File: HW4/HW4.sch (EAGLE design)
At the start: 27 parts

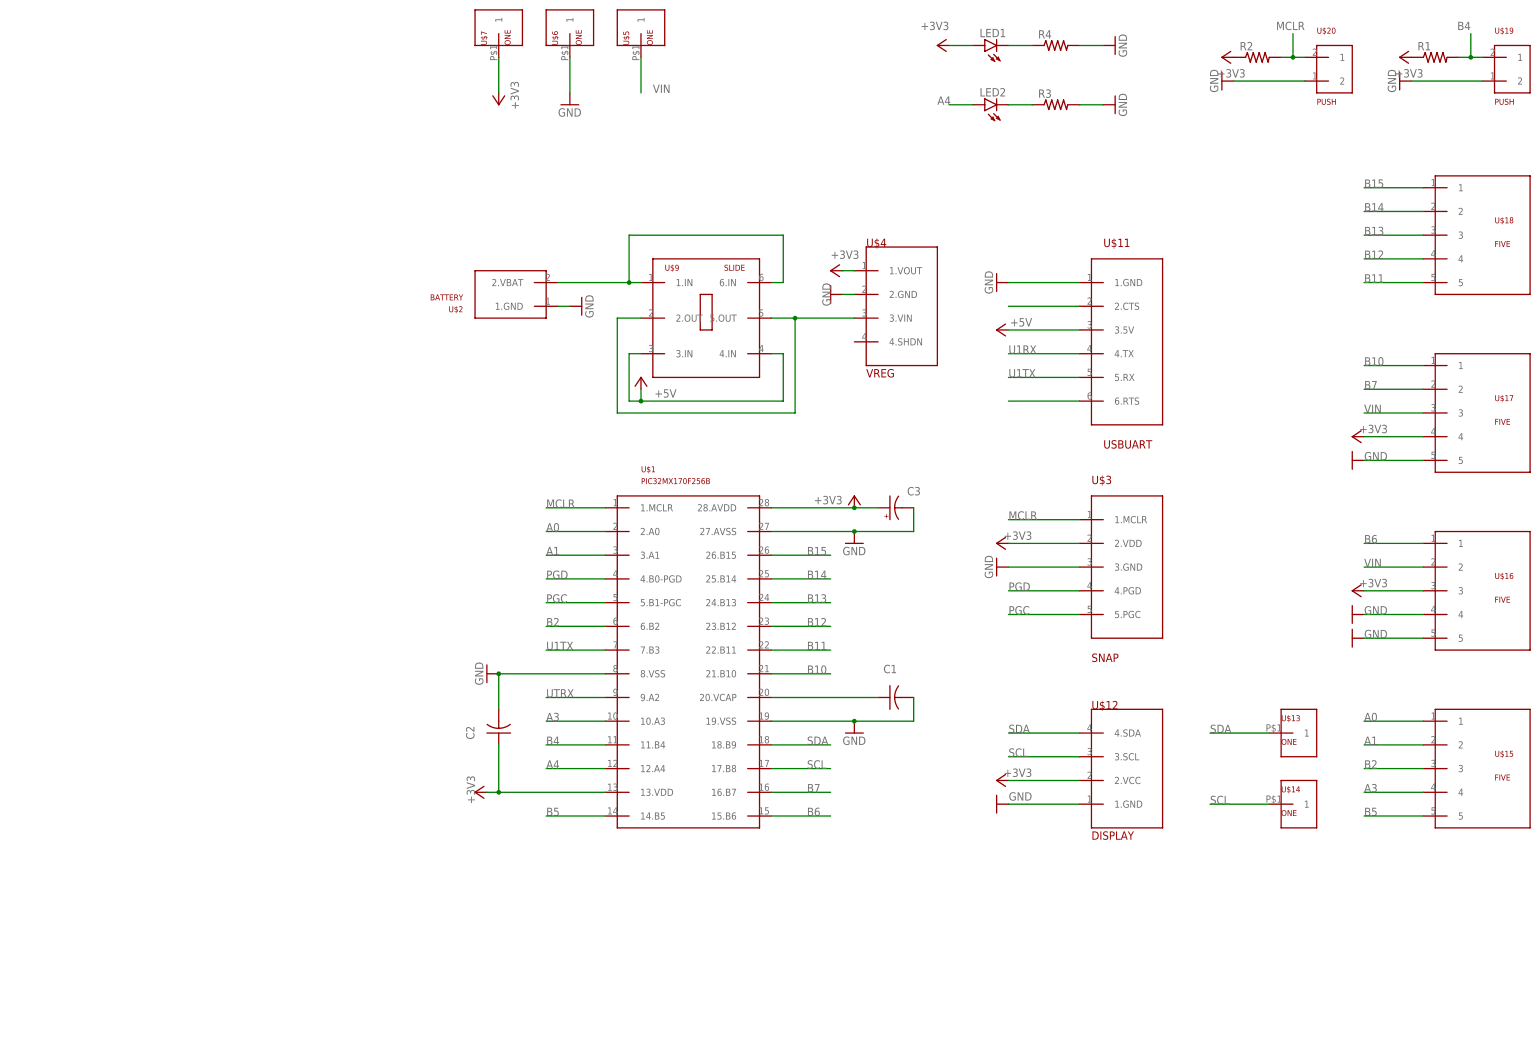
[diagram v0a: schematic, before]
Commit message: hw4 board/schematic update (finish)
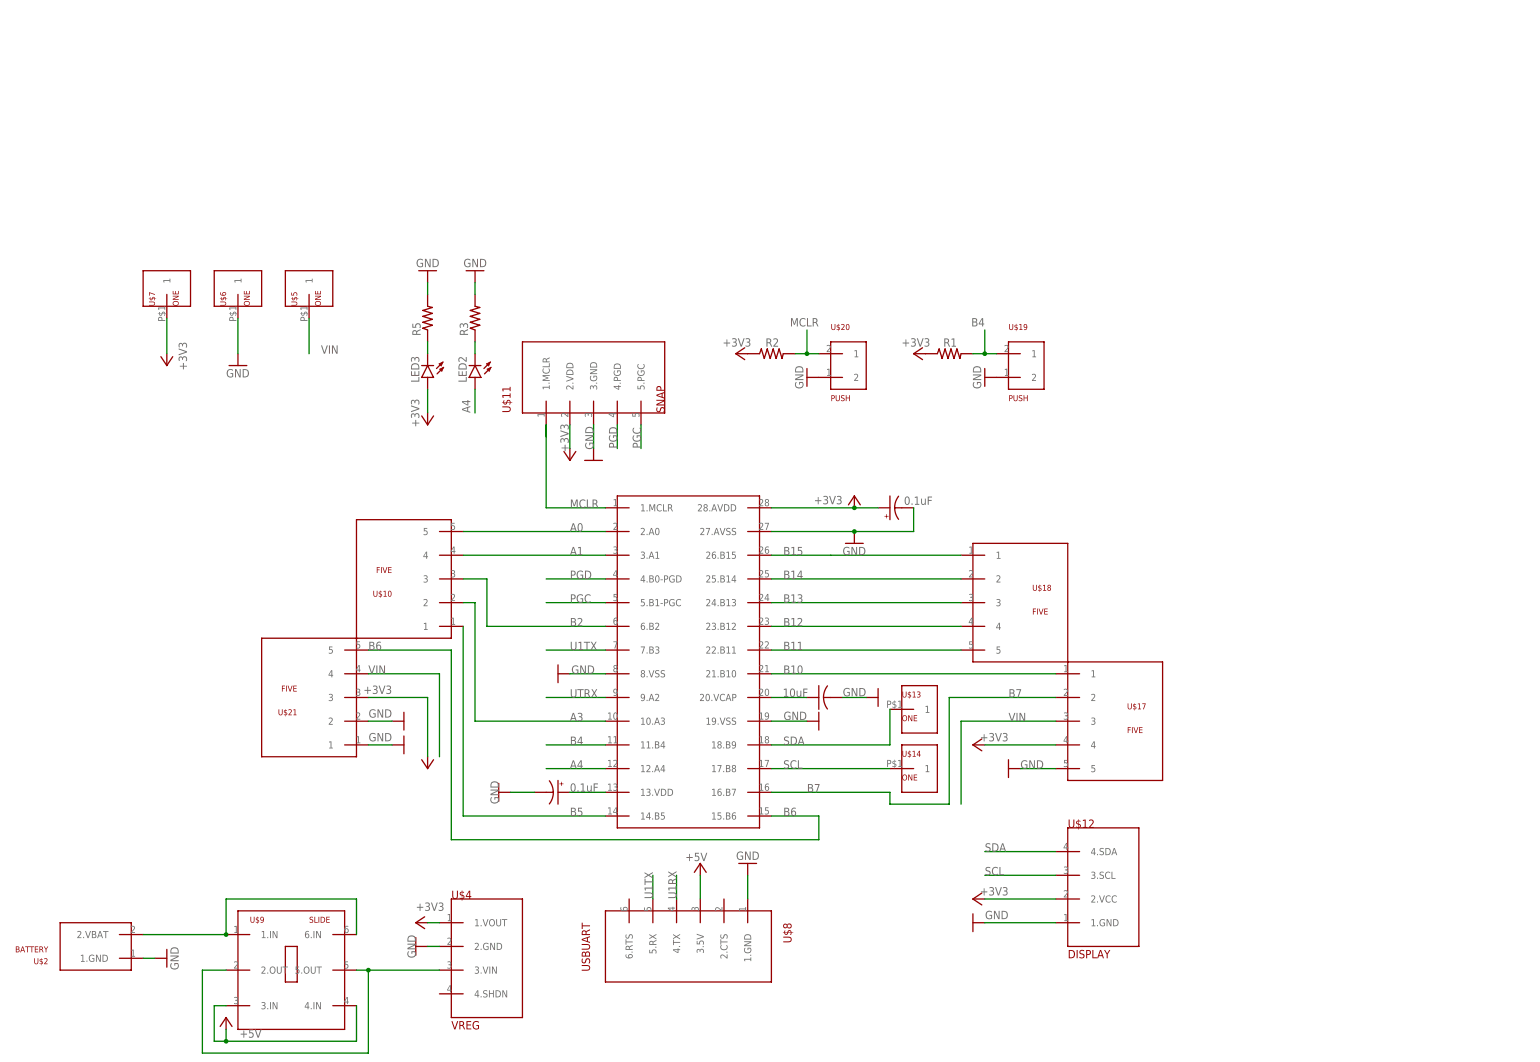
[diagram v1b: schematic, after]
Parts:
- removed LED1: (no value), HW4:LED3MM
- removed R4: (no value), HW4:R-US_0207/7
- removed U$15, U$16: FIVE, HW4:FIVE
- removed U$3: SNAP, HW4:SNAP
- added LED3: (no value), HW4:LED3MM
- added R5: (no value), HW4:R-US_0207/7
- added U$10, U$21: FIVE, HW4:FIVE
- added U$8: USBUART, HW4:USBUART
- C1: value (none) -> 10uF
- C2: value (none) -> 0.1uF; device HW4:C-US025-030X050 -> HW4:CPOL-USB45181B
- C3: value (none) -> 0.1uF
- U$11: value USBUART -> SNAP; device HW4:USBUART -> HW4:SNAP
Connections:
- removed net N$10: U$11.2.CTS
- removed net N$12: LED1.C, R4.1
- removed net N$6: U$11.6.RTS
- new net N$1: C2.+, U$1.13.VDD
- new net N$2: LED3.C, R5.1
- net +3V3: now also LED3.A, U$11.2.VDD, U$21.3; no longer C2.1, LED1.A, U$1.13.VDD, U$16.3, U$3.2.VDD
- net +5V: now also U$8.3.5V; no longer U$11.3.5V
- net A0: now also U$10.5; no longer U$15.1
- net A1: now also U$10.4; no longer U$15.2
- net A3: now also U$10.2; no longer U$15.4
- net B2: now also U$10.3; no longer U$15.3
- net B5: now also U$10.1; no longer U$15.5
- net B6: now also U$21.5; no longer U$16.1
- net GND: now also C2.-, R5.2, U$11.3.GND, U$21.1, U$21.2, U$8.1.GND; no longer C2.2, R4.2, U$11.1.GND, U$16.4, U$16.5, U$3.3.GND
- net MCLR: now also U$11.1.MCLR; no longer U$3.1.MCLR
- net PGC: now also U$11.5.PGC; no longer U$3.5.PGC
- net PGD: now also U$11.4.PGD; no longer U$3.4.PGD
- net U1RX: now also U$8.4.TX; no longer U$11.4.TX
- net U1TX: now also U$8.5.RX; no longer U$11.5.RX
- net VIN: now also U$21.4; no longer U$16.2
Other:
- moved on the sheet: LED2, R1, R2, R3, U$12, U$13, U$14, U$17, U$18, U$19, U$2, U$20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
